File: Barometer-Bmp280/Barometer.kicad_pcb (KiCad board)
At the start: 2 copper layers, 50 x 31 mm, 11 parts, among them J1 M80-8770405, U1 BMP280

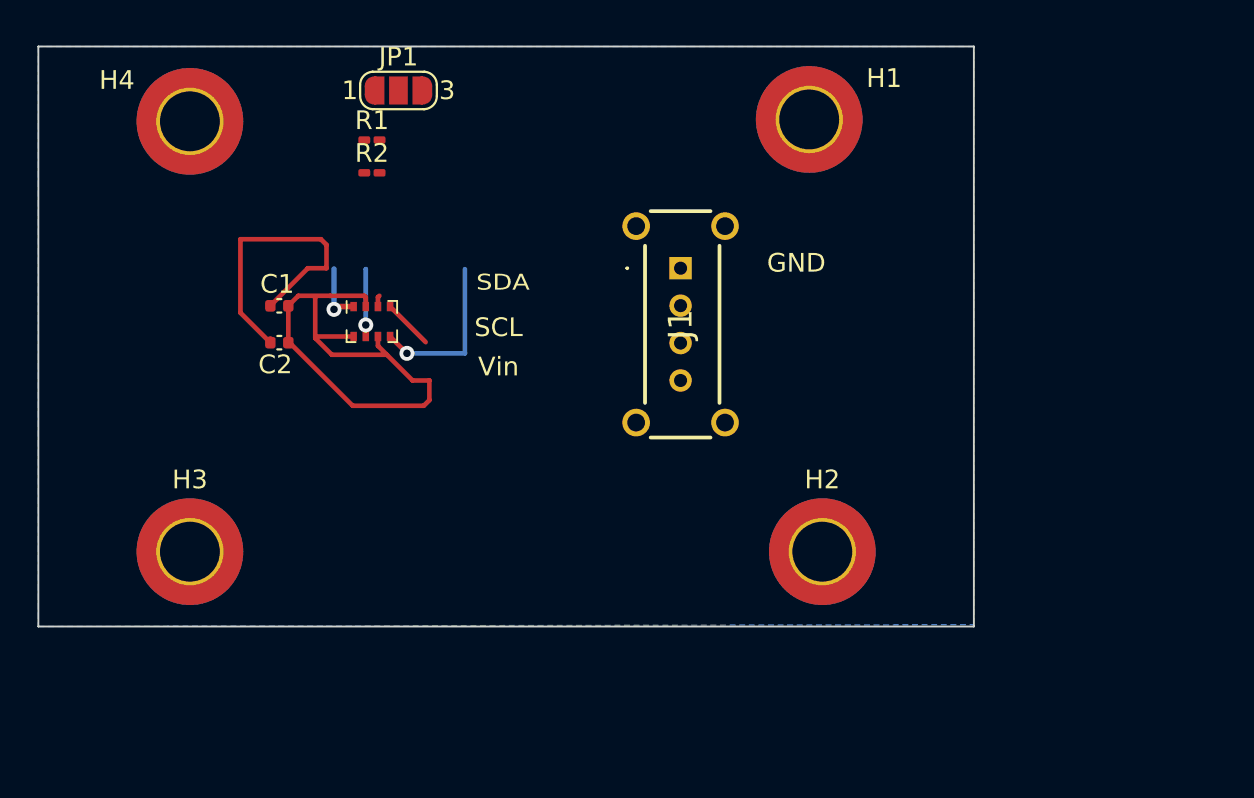
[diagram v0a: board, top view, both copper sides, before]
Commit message: LC24 PCBs
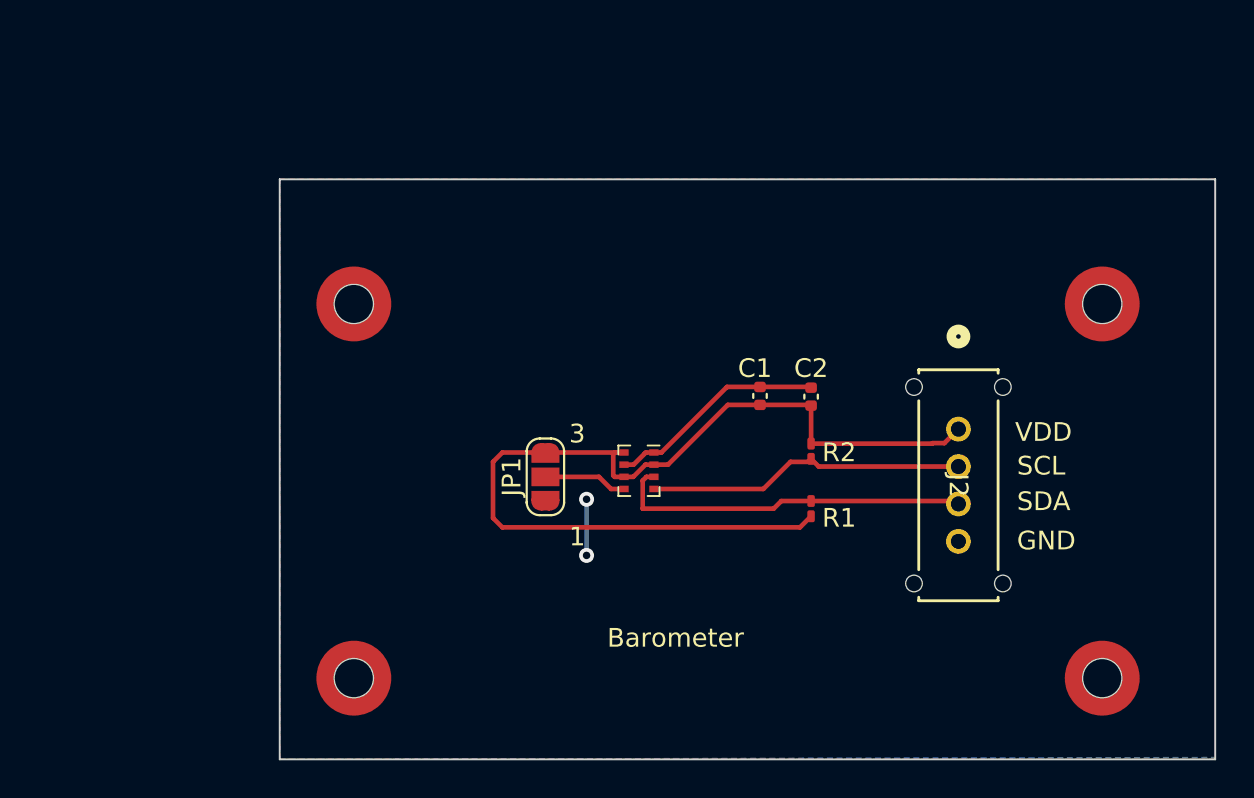
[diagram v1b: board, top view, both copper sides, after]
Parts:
- removed J1: M80-8770405, KiCad:M808770405
- added J2: M80-8770422, Harwin-M80-8770422:CONN_M80-87704_HRW, F.Cu at (136.3, 82.4)
- H1, H2, H3, H4: footprint MountingHole:MountingHole_3.2mm_M3_ISO7380_Pad_TopBottom -> Mounting_Wuerth:Mounting_Wuerth_WA-SMSI-M1.6_H1mm_9774010633
- moved H4 57.1 mm to (144.0, 95.7)
- moved H3 50.5 mm to (144.0, 75.7)
- moved H1 38.5 mm to (104.0, 95.7)
- moved R1 30.6 mm to (128.4, 86.6), turned to 90 degrees
- moved C2 28.6 mm to (128.4, 80.6), turned to 90 degrees
- moved H2 28.3 mm to (104.0, 75.7)
- moved R2 27.8 mm to (128.4, 83.5), turned to -90 degrees
- moved C1 26.1 mm to (125.7, 80.6), turned to 90 degrees
- moved JP1 22.1 mm to (114.2, 84.9), turned to 90 degrees
- moved U1 16.4 mm to (119.2, 84.6), turned to -90 degrees
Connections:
- JP1 pad 1: Net-(JP1-A) -> GND
- JP1 pad 2: +3.3V -> Net-(JP1-C)
- JP1 pad 3: GND -> +3.3V
- U1 pad 5: Net-(JP1-A) -> Net-(JP1-C)
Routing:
- net +3.3V: track 29.3 -> 52.1 mm
- net /SDA: track 0.61 -> 19.3 mm
- net /SCL: track 2.69 -> 17.1 mm
- net Net-(JP1-A): track 8.87 -> 0.00 mm, vias 1 -> 0
- net GND: track 23.2 -> 15.3 mm
- net Net-(JP1-C): track 0.00 -> 4.47 mm
- added copper zone on F.Cu, net GND
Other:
- board text added: "Barometer"
- board text added: "VDD"
- board text removed: "Vin"
